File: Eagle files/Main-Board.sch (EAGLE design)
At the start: 58 parts, among them J3 POWER_JACKPTH, J4 AVR_SPI_PRG_62X3_LOCK, Q1 DMN3404L, Q2 DMN3404L, Q3 DMN3404L, Q4 MMBT2222A, U1 ATMEGA328P, Y1 16mhz

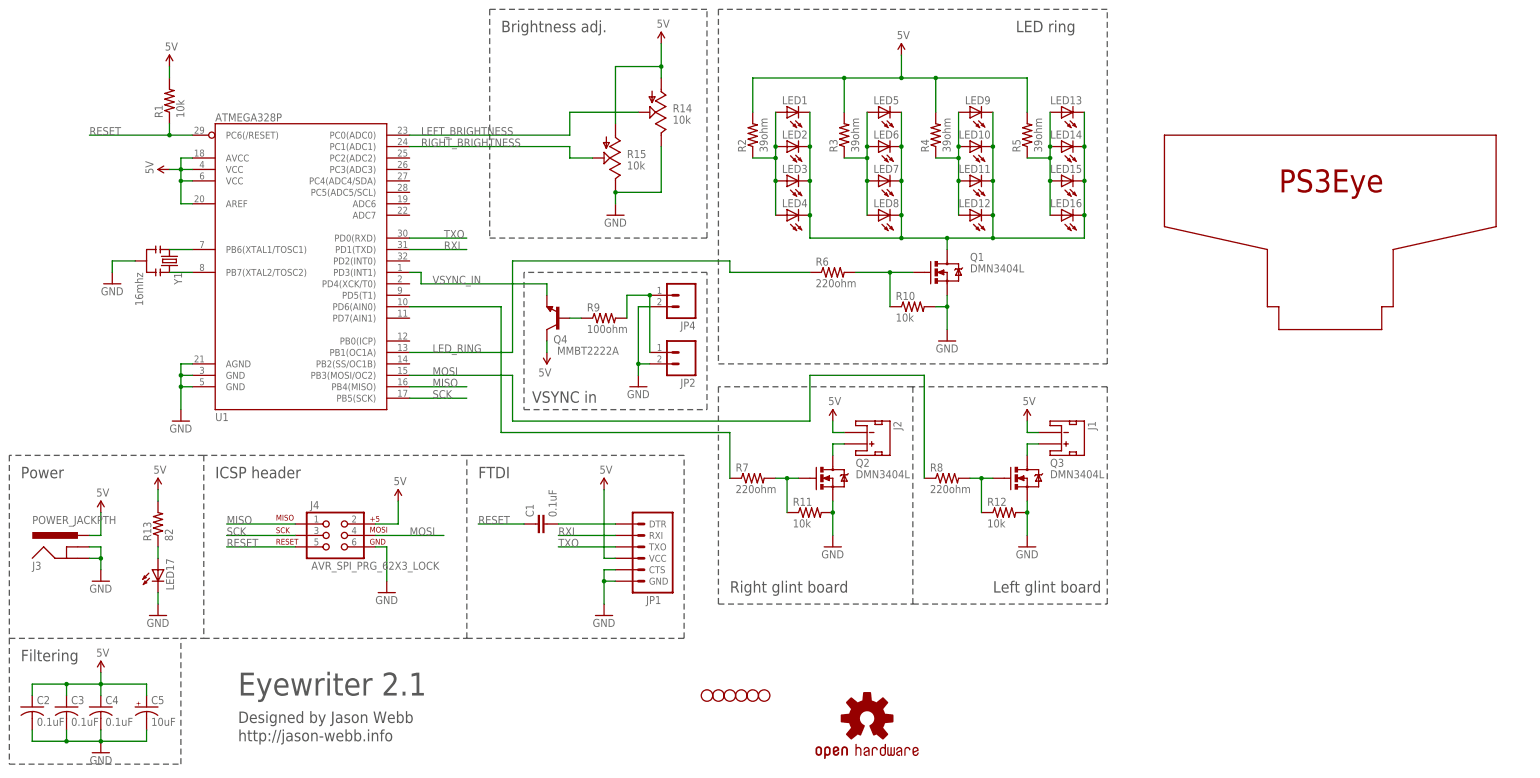
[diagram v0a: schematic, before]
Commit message: Updated Eagle files + BOMs
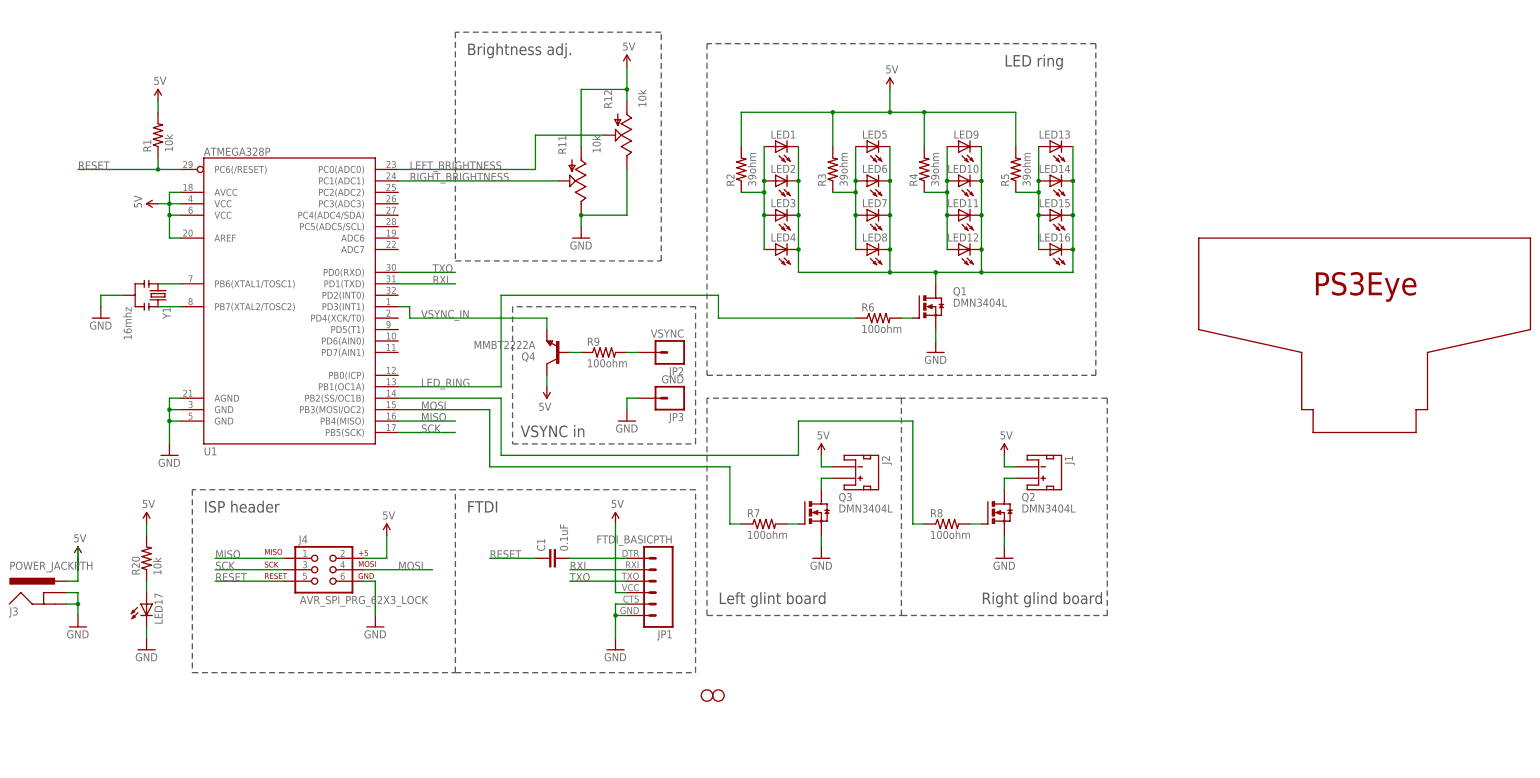
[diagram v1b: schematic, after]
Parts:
- removed C2, C3, C4: 0.1uF, adafruit:C-USC0805K
- removed C5: 10uF, adafruit:CPOL-USA/3216-18R
- removed JP4: (no value), SparkFun-Connectors:M02PTH
- removed LOGO1: OSHW-LOGOL, SparkFun-Aesthetics:OSHW-LOGOL
- removed R10: 10k, SparkFun-Resistors:RESISTOR0805-RES
- removed R13: 82, SparkFun-Resistors:RESISTOR0805-RES
- removed R14, R15: 10k, SparkFun-Electromechanical:POT
- removed STANDOFF3, STANDOFF4, STANDOFF5, STANDOFF6: STAND-OFF, SparkFun-Electromechanical:STAND-OFF
- removed U$1: PS3EYE, ps3eye:PS3EYE
- added JP3: GND, SparkFun-Connectors:M01PTH
- added R20: 10k, SparkFun-Resistors:RESISTOR0805-RES
- added U$4: PS3EYE, ps3eye:PS3EYE
- JP1: value (none) -> FTDI_BASICPTH; device SparkFun-Connectors:ARDUINO_SERIAL_PROGRAMLOCK -> SparkFun-Connectors:FTDI_BASICPTH
- JP2: value (none) -> VSYNC; device SparkFun-Connectors:M02PTH -> SparkFun-Connectors:M01PTH
- Q1, Q2, Q3: device SparkFun-DiscreteSemi:MOSFET-NCHANNELSMD -> transistor-power:N-HEXFET_SOT323-
- R11, R12: device SparkFun-Resistors:RESISTOR0805-RES -> SparkFun-Electromechanical:POT
- R6, R7, R8: value 220ohm -> 100ohm
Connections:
- removed net N$12: JP2.1, JP4.1, R9.2
- new net N$17: JP2.1, R9.2
- net 5V: now also JP1.4, R11.A, R12.A, R20.2; no longer C2.1, C3.1, C4.1, C5.+, JP1.VCC, R13.2, R14.A, R15.A
- net GLINT_RIGHT: now also U1.PB2(SS/OC1B); no longer U1.PB3(MOSI/OC2)
- net GND: now also JP1.5, JP1.6, JP3.1, R11.E, R12.E; no longer C2.2, C3.2, C4.2, C5.-, JP1.CTS, JP1.GND, JP2.2, JP4.2, R10.2, R11.2, R12.2, R14.E, R15.E
- net LEFT_BRIGHTNESS: now also R12.S; no longer R14.S
- net MOSI: now also U1.PB3(MOSI/OC2); no longer U1.PD6(AIN0)
- net N$1: now also R20.1; no longer R13.1
- net N$11: now also Q2.D; no longer Q3.D
- net N$14: now also Q2.G; no longer Q3.G, R12.1
- net N$16: now also JP1.1; no longer JP1.DTR
- net N$5: now also Q3.D; no longer Q2.D
- net N$7: no longer R10.1
- net N$9: now also Q3.G; no longer Q2.G, R11.1
- net RIGHT_BRIGHTNESS: now also R11.S; no longer R15.S
- net RXI: now also JP1.2; no longer JP1.RXI
- net TXO: now also JP1.3; no longer JP1.TXO
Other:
- note added: "ISP header"
- note added: "Right glind board"
- note removed: "Designed by Jason Webb"
- note removed: "Eyewriter 2.1"
- note removed: "Filtering"
- note removed: "ICSP header"
- note removed: "Power"
- note removed: "Right glint board"
- note removed: "http://jason-webb.info"
- moved on the sheet: C1, J1, J2, J3, J4, JP1, LED1, LED10, LED11, LED12, LED13, LED14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

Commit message: Updated Eagle files, including Gerbers and custom library
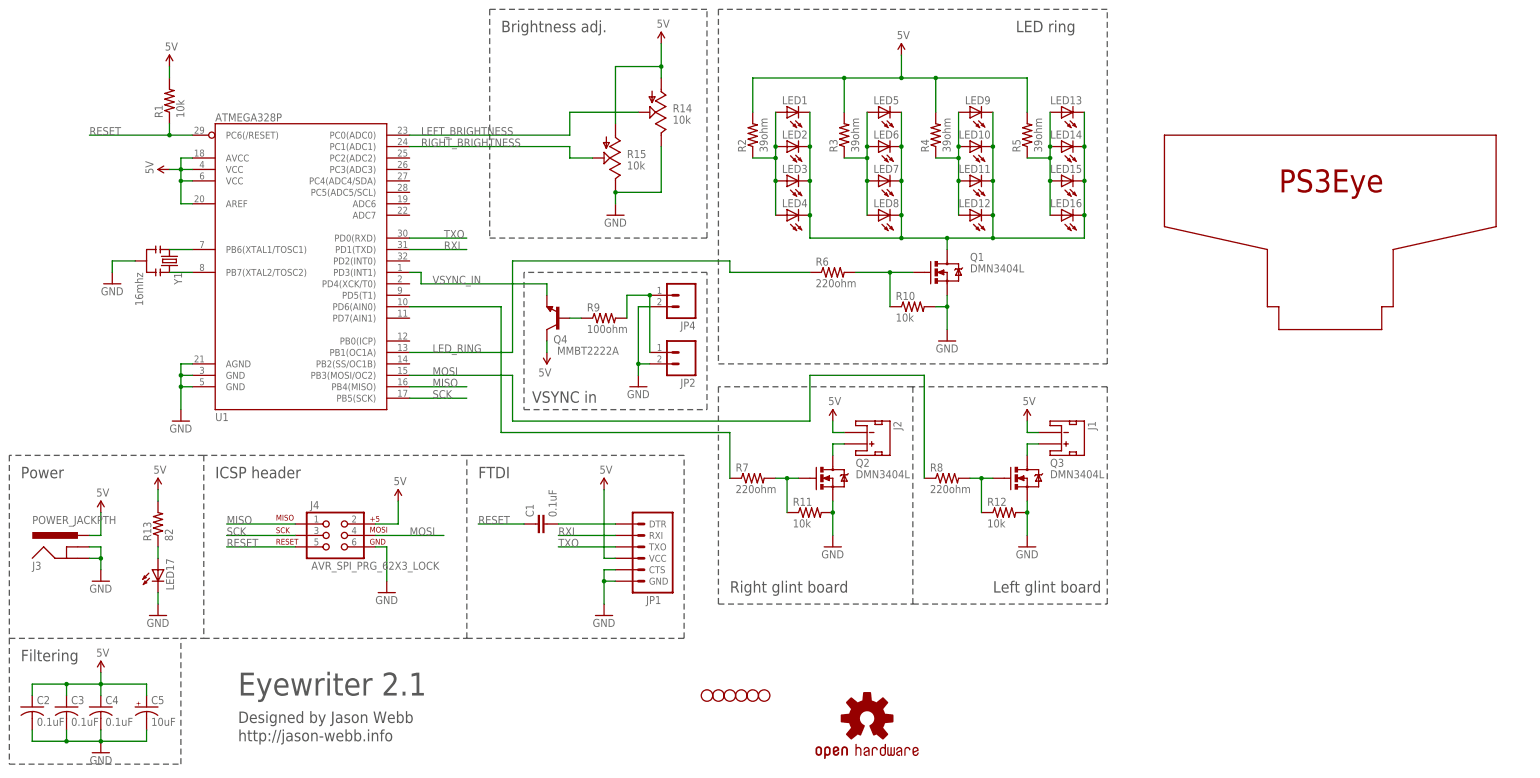
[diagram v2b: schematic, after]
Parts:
- removed JP3: GND, SparkFun-Connectors:M01PTH
- removed R20: 10k, SparkFun-Resistors:RESISTOR0805-RES
- removed U$4: PS3EYE, ps3eye:PS3EYE
- added C2, C3, C4: 0.1uF, adafruit:C-USC0805K
- added C5: 10uF, adafruit:CPOL-USA/3216-18R
- added JP4: (no value), SparkFun-Connectors:M02PTH
- added LOGO1: OSHW-LOGOL, SparkFun-Aesthetics:OSHW-LOGOL
- added R10: 10k, SparkFun-Resistors:RESISTOR0805-RES
- added R13: 82, SparkFun-Resistors:RESISTOR0805-RES
- added R14, R15: 10k, SparkFun-Electromechanical:POT
- added STANDOFF3, STANDOFF4, STANDOFF5, STANDOFF6: STAND-OFF, SparkFun-Electromechanical:STAND-OFF
- added U$1: PS3EYE, ps3eye:PS3EYE
- JP1: value FTDI_BASICPTH -> (none); device SparkFun-Connectors:FTDI_BASICPTH -> SparkFun-Connectors:ARDUINO_SERIAL_PROGRAMLOCK
- JP2: value VSYNC -> (none); device SparkFun-Connectors:M01PTH -> SparkFun-Connectors:M02PTH
- Q1, Q2, Q3: device transistor-power:N-HEXFET_SOT323- -> SparkFun-DiscreteSemi:MOSFET-NCHANNELSMD
- R11, R12: device SparkFun-Electromechanical:POT -> SparkFun-Resistors:RESISTOR0805-RES
- R6, R7, R8: value 100ohm -> 220ohm
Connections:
- removed net N$17: JP2.1, R9.2
- new net N$12: JP2.1, JP4.1, R9.2
- net 5V: now also C2.1, C3.1, C4.1, C5.+, JP1.VCC, R13.2, R14.A, R15.A; no longer JP1.4, R11.A, R12.A, R20.2
- net GLINT_RIGHT: now also U1.PB3(MOSI/OC2); no longer U1.PB2(SS/OC1B)
- net GND: now also C2.2, C3.2, C4.2, C5.-, JP1.CTS, JP1.GND, JP2.2, JP4.2, R10.2, R11.2, R12.2, R14.E, R15.E; no longer JP1.5, JP1.6, JP3.1, R11.E, R12.E
- net LEFT_BRIGHTNESS: now also R14.S; no longer R12.S
- net MOSI: now also U1.PD6(AIN0); no longer U1.PB3(MOSI/OC2)
- net N$1: now also R13.1; no longer R20.1
- net N$11: now also Q3.D; no longer Q2.D
- net N$14: now also Q3.G, R12.1; no longer Q2.G
- net N$16: now also JP1.DTR; no longer JP1.1
- net N$5: now also Q2.D; no longer Q3.D
- net N$7: now also R10.1
- net N$9: now also Q2.G, R11.1; no longer Q3.G
- net RIGHT_BRIGHTNESS: now also R15.S; no longer R11.S
- net RXI: now also JP1.RXI; no longer JP1.2
- net TXO: now also JP1.TXO; no longer JP1.3
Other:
- note added: "Designed by Jason Webb"
- note added: "Eyewriter 2.1"
- note added: "Filtering"
- note added: "ICSP header"
- note added: "Power"
- note added: "Right glint board"
- note added: "http://jason-webb.info"
- note removed: "ISP header"
- note removed: "Right glind board"
- moved on the sheet: C1, J1, J2, J3, J4, JP1, LED1, LED10, LED11, LED12, LED13, LED14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
